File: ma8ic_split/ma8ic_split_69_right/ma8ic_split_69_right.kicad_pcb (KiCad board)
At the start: 2 copper layers, 166.3 x 125.7 mm, 133 parts, among them J1 USB_C_Receptacle, J2 MJ-4PP-9, J3 I2C, J4 SPI, SW1 SW_PUSH, SW10 SW_PUSH-kbd, SW11 SW_PUSH-kbd, SW12 SW_PUSH-kbd, SW13 SW_PUSH-kbd, SW14 SW_PUSH-kbd, SW15 SW_PUSH-kbd, SW16 SW_PUSH-kbd, SW17 SW_PUSH-kbd, SW18 SW_PUSH-kbd, SW19 SW_PUSH-kbd, SW2 SW_PUSH-kbd, SW20 SW_PUSH-kbd, SW21 SW_PUSH-kbd, SW22 SW_PUSH-kbd, SW23 SW_PUSH-kbd, SW24 SW_PUSH-kbd, SW25 SW_PUSH-kbd, SW26 SW_PUSH-kbd, SW27 SW_PUSH-kbd, SW28 SW_PUSH-kbd, SW29 SW_PUSH-kbd, SW3 SW_PUSH-kbd, SW30 SW_PUSH-kbd, SW31 SW_PUSH-kbd, SW32 SW_PUSH-kbd, SW33 SW_PUSH-kbd, SW4 SW_PUSH-kbd, SW5 SW_PUSH-kbd, SW6 SW_PUSH-kbd, SW7 SW_PUSH-kbd, SW8 SW_PUSH-kbd, SW9 SW_PUSH-kbd, U1 ATMEGA32U4, X1 CSTNE16M0V530000R0

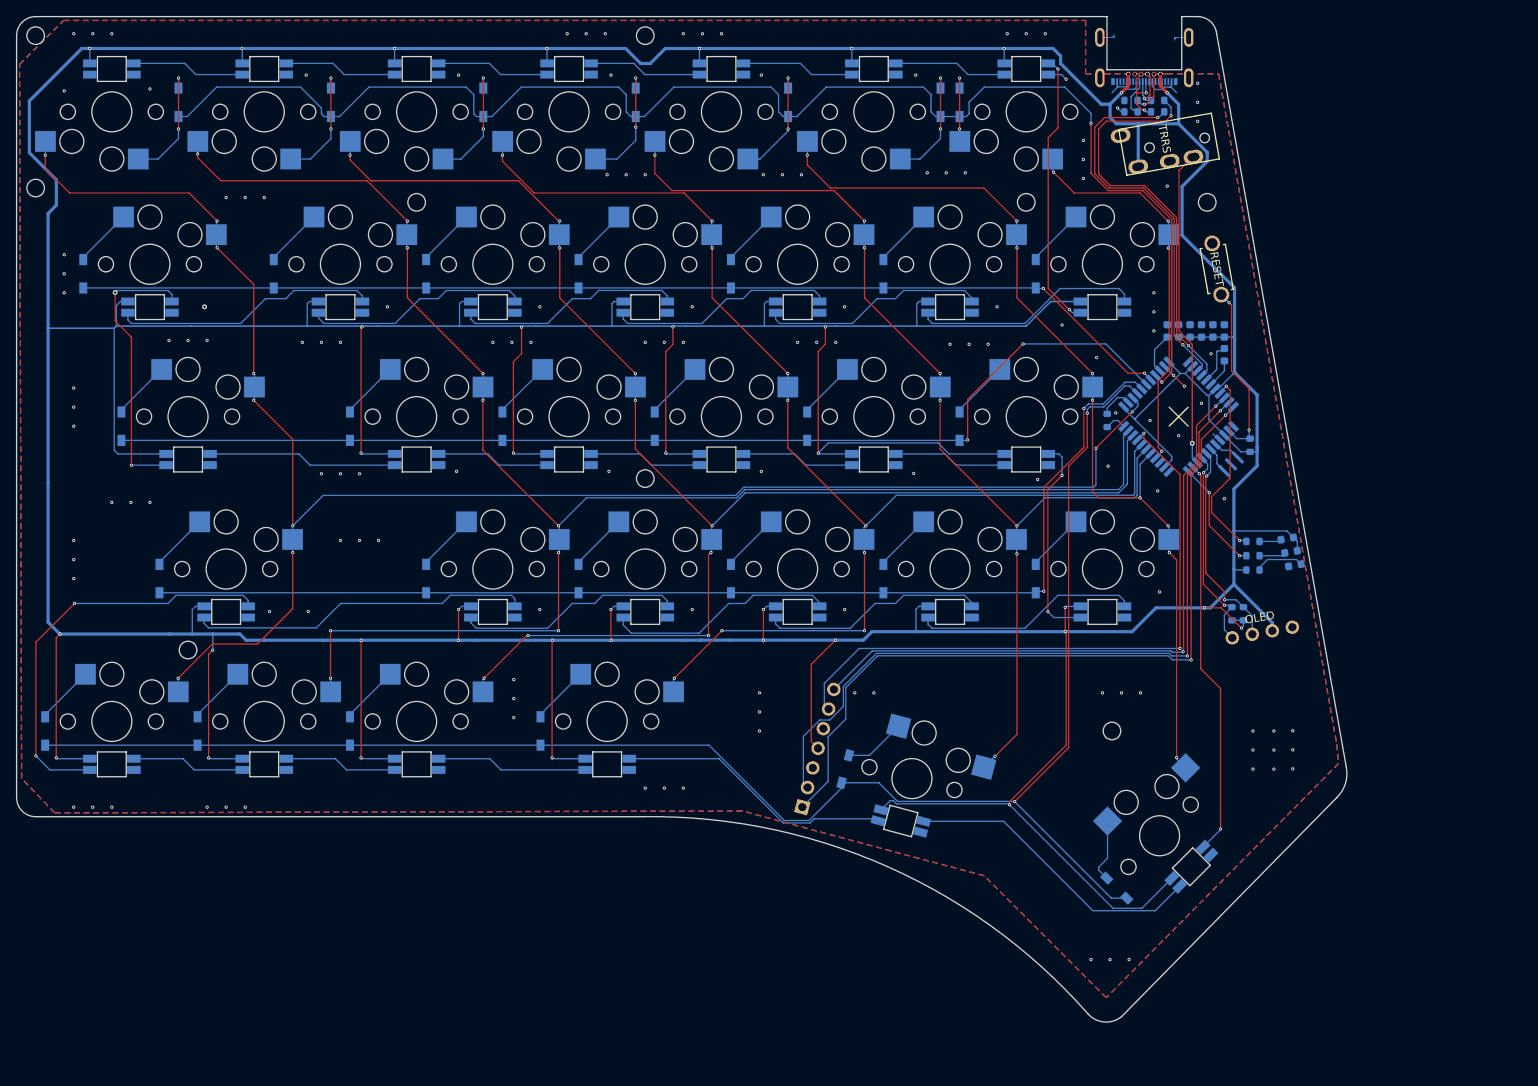
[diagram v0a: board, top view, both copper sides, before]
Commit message: update
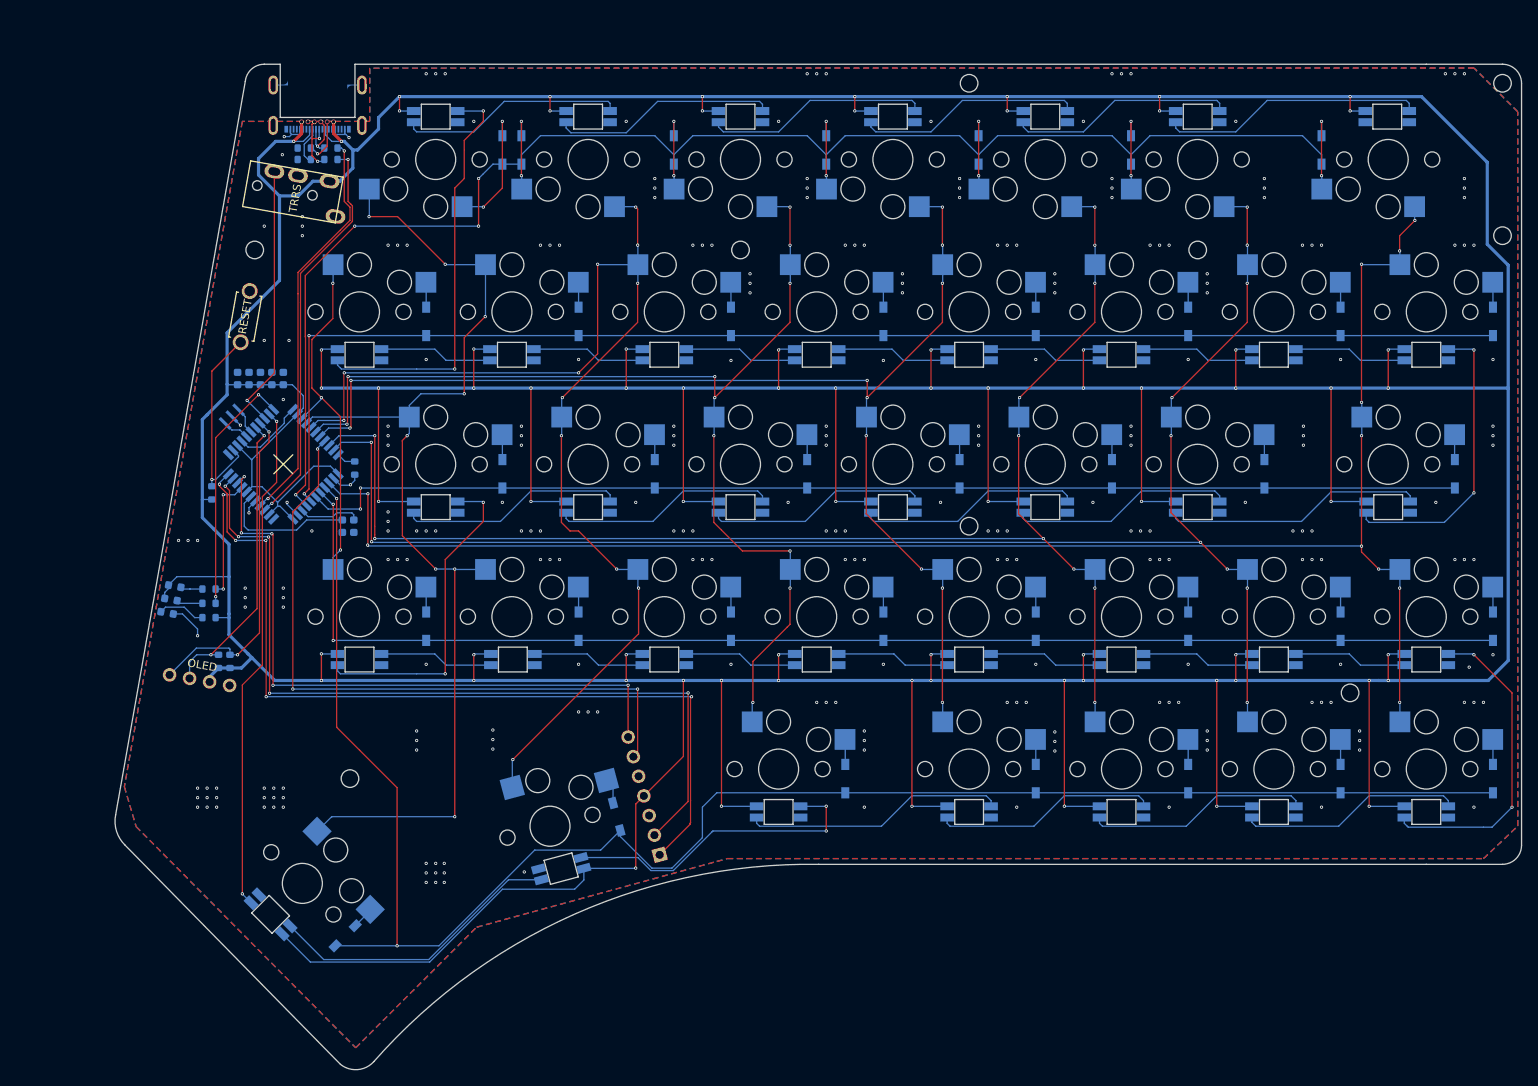
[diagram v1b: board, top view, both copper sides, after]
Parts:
- added D18: D_Small, ma8ic_split_69:D3_SMD_v2, B.Cu at (98.8, 67.9)
- added D25: D_Small, ma8ic_split_69:D3_SMD_v2, B.Cu at (108.3, 86.9)
- added D32: D_Small, ma8ic_split_69:D3_SMD_v2, B.Cu at (117.9, 106.0)
- added D33: D_Small, ma8ic_split_69:D3_SMD_v2, B.Cu at (98.8, 106.0)
- added D40: D_Small, ma8ic_split_69:D3_SMD_v2, B.Cu at (88.7, 144.7)
- added D55: SK6812MINI, ma8ic_split_69:YS-SK6812MINI-E, B.Cu at (90.5, 110.1)
- added D62: SK6812MINI, ma8ic_split_69:YS-SK6812MINI-E, B.Cu at (219.1, 91.1)
- added D69: SK6812MINI, ma8ic_split_69:YS-SK6812MINI-E, B.Cu at (109.5, 72.0)
- added D70: SK6812MINI, ma8ic_split_69:YS-SK6812MINI-E, B.Cu at (90.5, 72.0)
- added D77: SK6812MINI, ma8ic_split_69:YS-SK6812MINI-E, B.Cu at (219.0, 42.3)
- added SW16: SW_PUSH-kbd, ma8ic_split_69:ChocV1_V2_Hotswap, F.Cu at (90.5, 66.7)
- added SW23: SW_PUSH-kbd, ma8ic_split_69:ChocV1_V2_Hotswap, F.Cu at (100.0, 85.7)
- added SW30: SW_PUSH-kbd, ma8ic_split_69:ChocV1_V2_Hotswap, F.Cu at (109.5, 104.8)
- added SW31: SW_PUSH-kbd, ma8ic_split_69:ChocV1_V2_Hotswap, F.Cu at (90.5, 104.8)
- added SW38: SW_PUSH-kbd, ma8ic_split_69:ChocV1_V2_Hotswap_2u, F.Cu at (83.3, 138.1)
- ? (x5), REF** (x4): moved to B.Cu
- SW10, SW11, SW12, SW13, SW14, SW15, SW3, SW4, SW5, SW6, SW7, SW8: footprint kbd:ChocV1_V2_Hotswap -> ma8ic_split_69:ChocV1_V2_Hotswap
- SW17: renamed from SW16; footprint kbd:ChocV1_V2_Hotswap_2u -> ma8ic_split_69:ChocV1_V2_Hotswap_1.5u
- SW18: renamed from SW17; footprint kbd:ChocV1_V2_Hotswap -> ma8ic_split_69:ChocV1_V2_Hotswap
- SW19: renamed from SW18; footprint kbd:ChocV1_V2_Hotswap -> ma8ic_split_69:ChocV1_V2_Hotswap
- SW2: footprint kbd:ChocV1_V2_Hotswap -> ma8ic_split_69:ChocV1_V2_Hotswap_1.5u
- SW20: renamed from SW19; footprint kbd:ChocV1_V2_Hotswap -> ma8ic_split_69:ChocV1_V2_Hotswap
- SW21: renamed from SW20; footprint kbd:ChocV1_V2_Hotswap -> ma8ic_split_69:ChocV1_V2_Hotswap
- SW22: renamed from SW21; footprint kbd:ChocV1_V2_Hotswap -> ma8ic_split_69:ChocV1_V2_Hotswap
- SW24: renamed from SW22; footprint kbd:ChocV1_V2_Hotswap_2.5u -> ma8ic_split_69:ChocV1_V2_Hotswap
- SW25: renamed from SW23; footprint kbd:ChocV1_V2_Hotswap -> ma8ic_split_69:ChocV1_V2_Hotswap
- SW26: renamed from SW24; footprint kbd:ChocV1_V2_Hotswap -> ma8ic_split_69:ChocV1_V2_Hotswap
- SW27: renamed from SW25; footprint kbd:ChocV1_V2_Hotswap -> ma8ic_split_69:ChocV1_V2_Hotswap
- SW28: renamed from SW26; footprint kbd:ChocV1_V2_Hotswap -> ma8ic_split_69:ChocV1_V2_Hotswap
- SW29: renamed from SW27; footprint kbd:ChocV1_V2_Hotswap -> ma8ic_split_69:ChocV1_V2_Hotswap
- SW32: renamed from SW28; footprint kbd:ChocV1_V2_Hotswap -> ma8ic_split_69:ChocV1_V2_Hotswap
- SW33: renamed from SW29; footprint kbd:ChocV1_V2_Hotswap -> ma8ic_split_69:ChocV1_V2_Hotswap
- SW34: renamed from SW30; footprint kbd:ChocV1_V2_Hotswap -> ma8ic_split_69:ChocV1_V2_Hotswap
- SW35: renamed from SW31; footprint kbd:ChocV1_V2_Hotswap_1.5u -> ma8ic_split_69:ChocV1_V2_Hotswap
- SW36: renamed from SW32; footprint kbd:ChocV1_V2_Hotswap -> ma8ic_split_69:ChocV1_V2_Hotswap_1.5u
- SW37: renamed from SW33; footprint kbd:ChocV1_V2_Hotswap_2u -> ma8ic_split_69:ChocV1_V2_Hotswap
- SW9: footprint kbd:ChocV1_V2_Hotswap_1.5u -> ma8ic_split_69:ChocV1_V2_Hotswap
- moved ? 183.5 mm to (233.4, 38.1), turned to 180 degrees
- moved ? 183.5 mm to (233.4, 57.1), turned to 180 degrees
- moved D34 181.1 mm to (232.2, 125.0)
- moved D11 176.3 mm to (232.2, 67.9)
- moved D26 166.8 mm to (232.2, 106.0)
- moved D19 166.8 mm to (227.4, 86.9)
- moved SW32 164.4 mm to (223.8, 123.8)
- moved SW2 159.7 mm to (219.1, 47.6)
- moved SW9 159.7 mm to (223.8, 66.7)
- moved D47 152.1 mm to (223.8, 129.2)
- moved SW17 150.1 mm to (219.1, 85.7)
- moved SW24 150.1 mm to (223.8, 104.8)
- moved D46 145.4 mm to (204.8, 129.2)
- moved REF** 145.4 mm to (214.3, 114.3), turned to 180 degrees
- moved D4 143.0 mm to (210.7, 46.4)
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- renumbered D18 to D19, D19 to D20, D20 to D21, D21 to D22, D22 to D23, D23 to D24, D24 to D26, D25 to D27, D26 to D28, D27 to D29, D28 to D30, D29 to D31, D30 to D34, D31 to D35, D32 to D36, D33 to D37, D34 to D38, D35 to D39, D36 to D41, D37 to D42, D38 to D43, D39 to D44, D40 to D45, D41 to D46, D42 to D47, D43 to D48, D44 to D49, D45 to D50, D46 to D51, D47 to D52, D48 to D53, D49 to D54, D50 to D56, D51 to D57, D52 to D58, D53 to D59, D54 to D60, D55 to D61, D56 to D63, D57 to D64, D58 to D65, D59 to D66, D60 to D67, D61 to D68, D62 to D71, D63 to D72, D64 to D73, D65 to D74, D66 to D75, D67 to D76
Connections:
- D19 pad 2: Net-(D18-Pad2) -> Net-(D19-Pad2)
- D20 pad 2: Net-(D19-Pad2) -> Net-(D20-Pad2)
- D21 pad 2: Net-(D20-Pad2) -> Net-(D21-Pad2)
- D22 pad 2: Net-(D21-Pad2) -> Net-(D22-Pad2)
- D23 pad 2: Net-(D22-Pad2) -> Net-(D23-Pad2)
- D24 pad 2: Net-(D23-Pad2) -> Net-(D24-Pad2)
- D26 pad 2: Net-(D24-Pad2) -> Net-(D26-Pad2)
- D27 pad 2: Net-(D25-Pad2) -> Net-(D27-Pad2)
- D28 pad 2: Net-(D26-Pad2) -> Net-(D28-Pad2)
- D29 pad 2: Net-(D27-Pad2) -> Net-(D29-Pad2)
- D30 pad 2: Net-(D28-Pad2) -> Net-(D30-Pad2)
- D31 pad 2: Net-(D29-Pad2) -> Net-(D31-Pad2)
- D34 pad 2: Net-(D30-Pad2) -> Net-(D34-Pad2)
- D35 pad 2: Net-(D31-Pad2) -> Net-(D35-Pad2)
- D36 pad 2: Net-(D32-Pad2) -> Net-(D36-Pad2)
- D37 pad 2: Net-(D33-Pad2) -> Net-(D37-Pad2)
- D38 pad 2: Net-(D34-Pad2) -> Net-(D38-Pad2)
- D39 pad 2: Net-(D35-Pad2) -> Net-(D39-Pad2)
- D54 pad 2: Net-(D49-Pad2) (its old number) -> Net-(D54-Pad2)
- D56 pad 4: Net-(D49-Pad2) (its old number) -> Net-(D55-Pad2)
- D61 pad 2: Net-(D55-Pad2) -> Net-(D61-Pad2)
- D63 pad 4: Net-(D55-Pad2) -> Net-(D62-Pad2)
- D68 pad 2: Net-(D61-Pad2) -> Net-(D68-Pad2)
- D71 pad 4: Net-(D61-Pad2) -> Net-(D70-Pad2)
- D76 pad 2: unconnected-(D67-Pad2) -> Net-(D76-Pad2)
- SW10 pad 1: COL1 -> Net-(D12-Pad2)
- SW10 pad 2: Net-(D12-Pad2) -> COL1
- SW11 pad 1: COL2 -> Net-(D13-Pad2)
- SW11 pad 2: Net-(D13-Pad2) -> COL2
- SW12 pad 1: COL3 -> Net-(D14-Pad2)
- SW12 pad 2: Net-(D14-Pad2) -> COL3
- SW13 pad 1: COL4 -> Net-(D15-Pad2)
- SW13 pad 2: Net-(D15-Pad2) -> COL4
- SW14 pad 1: COL5 -> Net-(D16-Pad2)
- SW14 pad 2: Net-(D16-Pad2) -> COL5
- SW15 pad 1: COL6 -> Net-(D17-Pad2)
- SW15 pad 2: Net-(D17-Pad2) -> COL6
- SW17 pad 1: COL0 -> Net-(D19-Pad2)
- SW17 pad 2: Net-(D18-Pad2) -> COL0
- SW18 pad 1: COL1 -> Net-(D20-Pad2)
- SW18 pad 2: Net-(D19-Pad2) -> COL1
- SW19 pad 1: COL2 -> Net-(D21-Pad2)
- SW19 pad 2: Net-(D20-Pad2) -> COL2
- SW2 pad 1: COL0 -> Net-(D4-Pad2)
- SW2 pad 2: Net-(D4-Pad2) -> COL0
- SW20 pad 1: COL3 -> Net-(D22-Pad2)
- SW20 pad 2: Net-(D21-Pad2) -> COL3
- SW21 pad 1: COL4 -> Net-(D23-Pad2)
- SW21 pad 2: Net-(D22-Pad2) -> COL4
- SW22 pad 1: COL5 -> Net-(D24-Pad2)
- SW22 pad 2: Net-(D23-Pad2) -> COL5
- SW24 pad 1: COL0 -> Net-(D26-Pad2)
- SW24 pad 2: Net-(D24-Pad2) -> COL0
- SW25 pad 1: COL1 -> Net-(D27-Pad2)
- SW25 pad 2: Net-(D25-Pad2) -> COL1
- SW26 pad 1: COL2 -> Net-(D28-Pad2)
- SW26 pad 2: Net-(D26-Pad2) -> COL2
- SW27 pad 1: COL3 -> Net-(D29-Pad2)
- SW27 pad 2: Net-(D27-Pad2) -> COL3
- SW28 pad 1: COL4 -> Net-(D30-Pad2)
- SW28 pad 2: Net-(D28-Pad2) -> COL4
- SW29 pad 1: COL5 -> Net-(D31-Pad2)
- SW29 pad 2: Net-(D29-Pad2) -> COL5
- SW3 pad 1: COL1 -> Net-(D5-Pad2)
- SW3 pad 2: Net-(D5-Pad2) -> COL1
- SW32 pad 1: COL0 -> Net-(D34-Pad2)
- SW32 pad 2: Net-(D30-Pad2) -> COL0
- SW33 pad 1: COL1 -> Net-(D35-Pad2)
- SW33 pad 2: Net-(D31-Pad2) -> COL1
- SW34 pad 1: COL2 -> Net-(D36-Pad2)
- SW34 pad 2: Net-(D32-Pad2) -> COL2
- SW35 pad 1: COL3 -> Net-(D37-Pad2)
- SW35 pad 2: Net-(D33-Pad2) -> COL3
- SW36 pad 1: COL4 -> Net-(D38-Pad2)
- SW36 pad 2: Net-(D34-Pad2) -> COL4
- SW37 pad 1: COL5 -> Net-(D39-Pad2)
- SW37 pad 2: Net-(D35-Pad2) -> COL5
- SW4 pad 1: COL2 -> Net-(D6-Pad2)
- SW4 pad 2: Net-(D6-Pad2) -> COL2
- SW5 pad 1: COL3 -> Net-(D7-Pad2)
- SW5 pad 2: Net-(D7-Pad2) -> COL3
- SW6 pad 1: COL4 -> Net-(D8-Pad2)
- SW6 pad 2: Net-(D8-Pad2) -> COL4
- SW7 pad 1: COL5 -> Net-(D9-Pad2)
- SW7 pad 2: Net-(D9-Pad2) -> COL5
- SW8 pad 1: Net-(D10-Pad2) -> COL6
- SW8 pad 2: COL6 -> Net-(D10-Pad2)
- SW9 pad 1: COL0 -> Net-(D11-Pad2)
- SW9 pad 2: Net-(D11-Pad2) -> COL0
- U1 pad 25: unconnected-(U1-Pad25) -> COL7
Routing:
- net VCC: track 1030.9 -> 1118.4 mm, vias 37 -> 74
- net COL6: track 49.4 -> 136.1 mm, vias 4 -> 8
- net Net-(D70-Pad2): track 0.00 -> 52.4 mm, vias 0 -> 2
- net COL7: track 0.00 -> 44.7 mm, vias 0 -> 3
- net Net-(D62-Pad2): track 0.00 -> 37.1 mm, vias 0 -> 2
- net COL5: track 118.4 -> 151.3 mm, vias 9 -> 12
- net Net-(D76-Pad2): track 0.00 -> 32.8 mm
- net ROW1: track 138.2 -> 169.3 mm
- net Net-(D46-Pad2): track 51.7 -> 27.9 mm, vias 2 -> 0
- net Net-(D67-Pad2): track 34.7 -> 14.1 mm, vias 2 -> 0
- net ROW3: track 144.5 -> 164.3 mm
- net Net-(D61-Pad2): track 14.1 -> 32.6 mm
- net Net-(R8-Pad2): track 14.3 -> 30.9 mm
- net SDA: track 25.7 -> 41.7 mm
- net Net-(D49-Pad2): track 28.7 -> 14.1 mm
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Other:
- board size 166.3 x 125.7 mm -> 175.8 x 125.7 mm
- board text added: "33"
- board text added: "34"
- board text added: "35"
- board text added: "36"
- board text added: "37"
- board text added: "driving="
- board text added: "hearing="
- board text added: "talking="
- board text removed: "=driving"
- board text removed: "=hearing"
- board text removed: "=talking"
